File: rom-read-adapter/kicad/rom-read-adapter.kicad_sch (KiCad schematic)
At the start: 51 parts, among them J1 Host_Conn_02x25, J10 Conn_01x04_Pin, J2 ZIF-48, J3 Conn_01x24_Pin, J4 Conn_01x13_Pin, J5 Conn_01x05_Pin

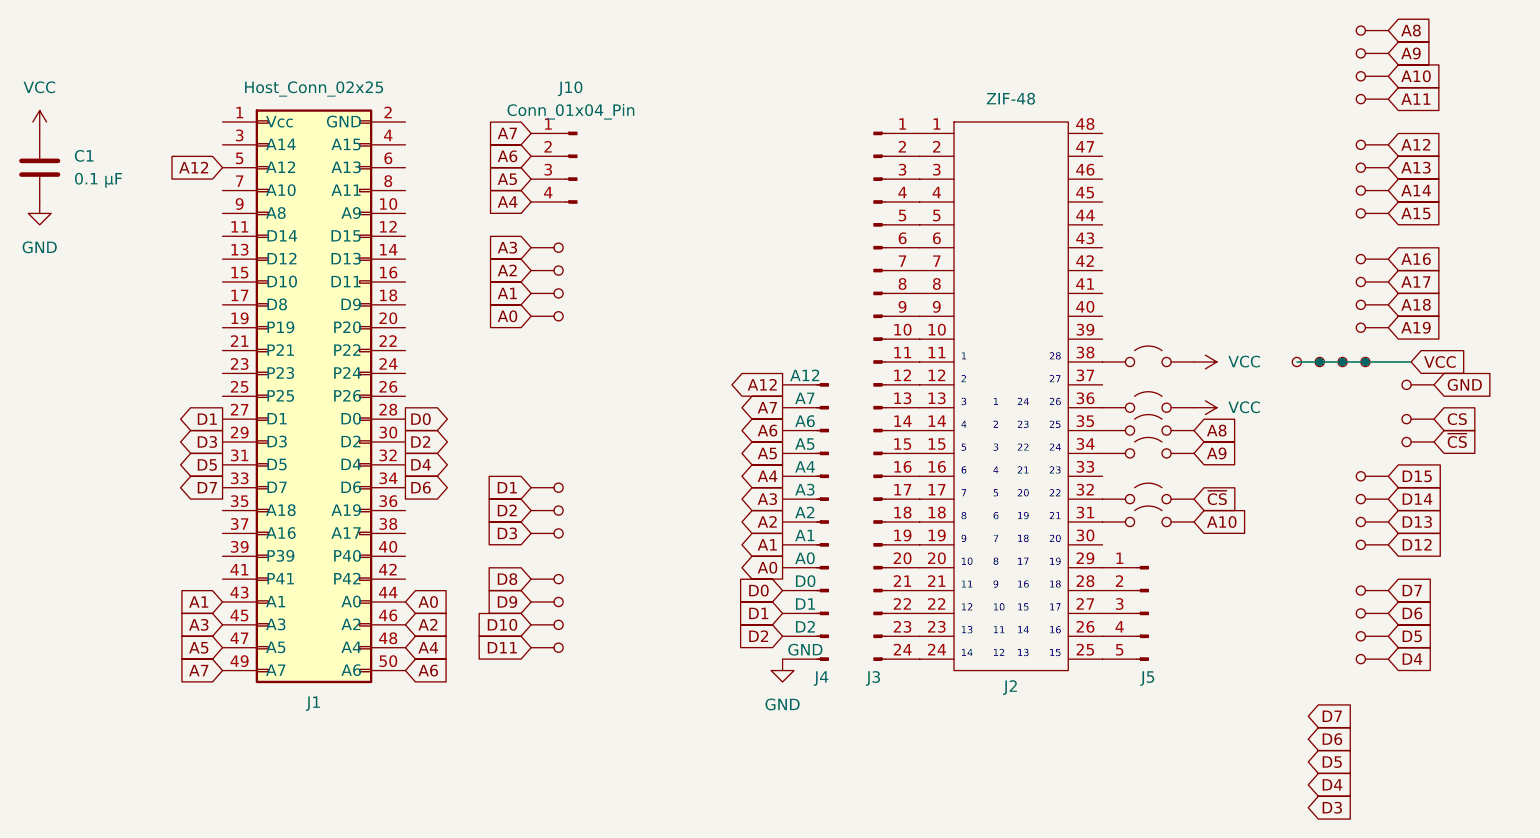
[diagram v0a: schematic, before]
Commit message: WIP rom-read-adapter sch: Added J6.
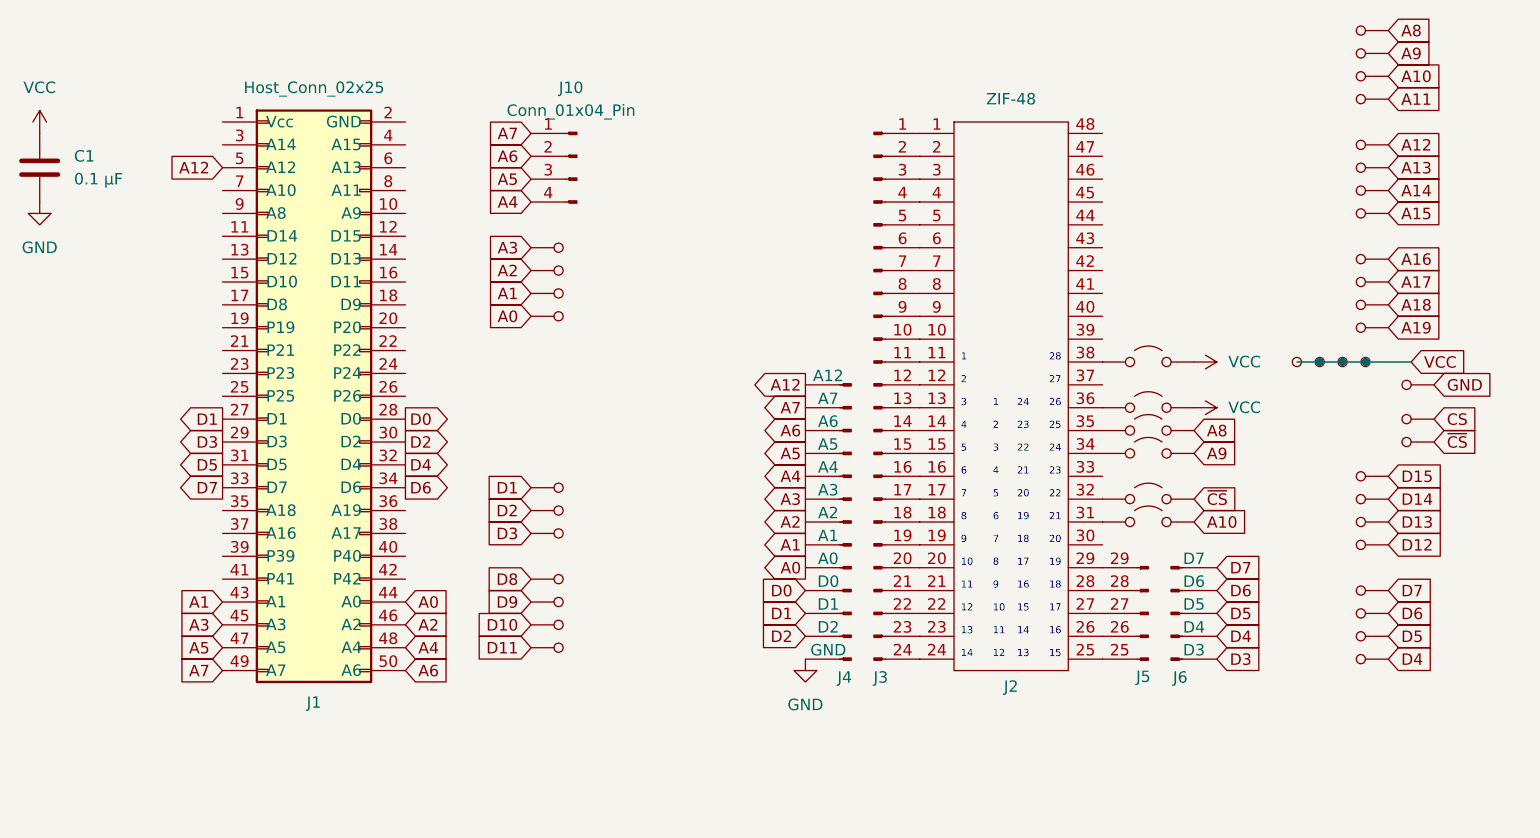
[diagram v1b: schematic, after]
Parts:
- added J6: Conn_01x05_Pin, symbol Connector:Conn_01x05_Pin
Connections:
- net D3: now also J6.1 (D3)
- net D4: now also J6.2 (D4)
- net D5: now also J6.3 (D5)
- net D6: now also J6.4 (D6)
- net D7: now also J6.5 (D7)
- net at J2., J2.28: now also J5.28 (Pin_4); no longer J5.2 (Pin_2)
- net at J2.25: now also J5.25 (Pin_1); no longer J5.5 (Pin_5)
- net at J2.26: now also J5.26 (Pin_2); no longer J5.4 (Pin_4)
- net at J2.27: now also J5.27 (Pin_3); no longer J5.3 (Pin_3)
- net at J2.29: now also J5.29 (Pin_5); no longer J5.1 (Pin_1)
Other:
- moved on the sheet: J4, J5
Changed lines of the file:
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@@
 	(global_label "A7"
 		(shape output)
-		(at 113.03 95.25 180)
+		(at 115.57 95.25 180)
 		(fields_autoplaced yes)
 		(effects
@@
 		)
 		(property "Intersheetrefs" "${INTERSHEET_REFS}"
-			(at 107.7467 95.25 0)
+			(at 110.2867 95.25 0)
 			(effects
 				(font
@@
 	(global_label "A2"
 		(shape output)
-		(at 113.03 107.95 180)
+		(at 115.57 107.95 180)
 		(fields_autoplaced yes)
 		(effects
@@
 		)
 		(property "Intersheetrefs" "${INTERSHEET_REFS}"
-			(at 107.7467 107.95 0)
+			(at 110.2867 107.95 0)
 			(effects
 				(font
@@
 	(global_label "D3"
 		(shape input)
-		(at 171.45 139.7 0)
+		(at 161.29 123.19 0)
 		(fields_autoplaced yes)
 		(effects
@@
 		)
 		(property "Intersheetrefs" "${INTERSHEET_REFS}"
-			(at 176.9147 139.7 0)
+			(at 166.7547 123.19 0)
 			(effects
 				(font
@@
 	(global_label "A12"
 		(shape output)
-		(at 113.03 92.71 180)
+		(at 115.57 92.71 180)
 		(fields_autoplaced yes)
 		(effects
@@
 		)
 		(property "Intersheetrefs" "${INTERSHEET_REFS}"
-			(at 106.5372 92.71 0)
+			(at 109.0772 92.71 0)
 			(effects
 				(font
@@
 	(global_label "D2"
 		(shape input)
-		(at 113.03 120.65 180)
+		(at 115.57 120.65 180)
 		(fields_autoplaced yes)
 		(effects
@@
 		)
 		(property "Intersheetrefs" "${INTERSHEET_REFS}"
-			(at 107.5653 120.65 0)
+			(at 110.1053 120.65 0)
 			(effects
 				(font
@@
 	(global_label "D1"
 		(shape input)
-		(at 113.03 118.11 180)
+		(at 115.57 118.11 180)
 		(fields_autoplaced yes)
 		(effects
@@
 		)
 		(property "Intersheetrefs" "${INTERSHEET_REFS}"
-			(at 107.5653 118.11 0)
+			(at 110.1053 118.11 0)
 			(effects
 				(font
@@
 	(global_label "A0"
 		(shape output)
-		(at 113.03 113.03 180)
+		(at 115.57 113.03 180)
 		(fields_autoplaced yes)
 		(effects
@@
 		)
 		(property "Intersheetrefs" "${INTERSHEET_REFS}"
-			(at 107.7467 113.03 0)
+			(at 110.2867 113.03 0)
 			(effects
 				(font
@@
 	(global_label "A5"
 		(shape output)
-		(at 113.03 100.33 180)
+		(at 115.57 100.33 180)
 		(fields_autoplaced yes)
 		(effects
@@
 		)
 		(property "Intersheetrefs" "${INTERSHEET_REFS}"
-			(at 107.7467 100.33 0)
+			(at 110.2867 100.33 0)
 			(effects
 				(font
@@
 	(global_label "D4"
 		(shape input)
-		(at 171.45 137.16 0)
+		(at 161.29 120.65 0)
 		(fields_autoplaced yes)
 		(effects
@@
 		)
 		(property "Intersheetrefs" "${INTERSHEET_REFS}"
-			(at 176.9147 137.16 0)
+			(at 166.7547 120.65 0)
 			(effects
 				(font
@@
 	(global_label "A1"
 		(shape output)
-		(at 113.03 110.49 180)
+		(at 115.57 110.49 180)
 		(fields_autoplaced yes)
 		(effects
@@
 		)
 		(property "Intersheetrefs" "${INTERSHEET_REFS}"
-			(at 107.7467 110.49 0)
+			(at 110.2867 110.49 0)
 			(effects
 				(font
@@
 	(global_label "A3"
 		(shape output)
-		(at 113.03 105.41 180)
+		(at 115.57 105.41 180)
 		(fields_autoplaced yes)
 		(effects
@@
 		)
 		(property "Intersheetrefs" "${INTERSHEET_REFS}"
-			(at 107.7467 105.41 0)
+			(at 110.2867 105.41 0)
 			(effects
 				(font
@@
 	(global_label "D5"
 		(shape input)
-		(at 171.45 134.62 0)
+		(at 161.29 118.11 0)
 		(fields_autoplaced yes)
 		(effects
@@
 		)
 		(property "Intersheetrefs" "${INTERSHEET_REFS}"
-			(at 176.9147 134.62 0)
+			(at 166.7547 118.11 0)
 			(effects
 				(font
@@
 	(global_label "A6"
 		(shape output)
-		(at 113.03 97.79 180)
+		(at 115.57 97.79 180)
 		(fields_autoplaced yes)
 		(effects
@@
 		)
 		(property "Intersheetrefs" "${INTERSHEET_REFS}"
-			(at 107.7467 97.79 0)
+			(at 110.2867 97.79 0)
 			(effects
 				(font
@@
 	(global_label "D6"
 		(shape input)
-		(at 171.45 132.08 0)
+		(at 161.29 115.57 0)
 		(fields_autoplaced yes)
 		(effects
@@
 		)
 		(property "Intersheetrefs" "${INTERSHEET_REFS}"
-			(at 176.9147 132.08 0)
+			(at 166.7547 115.57 0)
 			(effects
 				(font
@@
 	(global_label "D7"
 		(shape input)
-		(at 171.45 129.54 0)
+		(at 161.29 113.03 0)
 		(fields_autoplaced yes)
 		(effects
@@
 		)
 		(property "Intersheetrefs" "${INTERSHEET_REFS}"
-			(at 176.9147 129.54 0)
+			(at 166.7547 113.03 0)
 			(effects
 				(font
@@
 	(global_label "A4"
 		(shape output)
-		(at 113.03 102.87 180)
+		(at 115.57 102.87 180)
 		(fields_autoplaced yes)
 		(effects
@@
 		)
 		(property "Intersheetrefs" "${INTERSHEET_REFS}"
-			(at 107.7467 102.87 0)
+			(at 110.2867 102.87 0)
 			(effects
 				(font
@@
 	(global_label "D0"
 		(shape input)
-		(at 113.03 115.57 180)
+		(at 115.57 115.57 180)
 		(fields_autoplaced yes)
 		(effects
@@
 		)
 		(property "Intersheetrefs" "${INTERSHEET_REFS}"
-			(at 107.5653 115.57 0)
+			(at 110.1053 115.57 0)
 			(effects
 				(font
@@
 	(symbol
 		(lib_id "power:GND")
-		(at 113.03 123.19 0)
+		(at 115.57 123.19 0)
 		(unit 1)
 		(exclude_from_sim no)
@@
 		(fields_autoplaced yes)
 		(property "Reference" "#PWR03"
-			(at 113.03 129.54 0)
+			(at 115.57 129.54 0)
 			(effects
 				(font
@@
 		)
 		(property "Value" "GND"
-			(at 113.03 128.27 0)
+			(at 115.57 128.27 0)
 			(effects
 				(font
@@
 		)
 		(property "Footprint" ""
-			(at 113.03 123.19 0)
+			(at 115.57 123.19 0)
 			(effects
 				(font
@@
 		)
 		(property "Datasheet" ""
-			(at 113.03 123.19 0)
+			(at 115.57 123.19 0)
 			(effects
 				(font
@@
 		)
 		(property "Description" "Power symbol creates a global label with name \"GND\" , ground"
-			(at 113.03 123.19 0)
+			(at 115.57 123.19 0)
 			(effects
 				(font
@@
 	)
 	(symbol
+		(lib_name "Conn_01x05_Pin_1")
 		(lib_id "Connector:Conn_01x05_Pin")
-		(at 153.67 118.11 0)
-		(mirror y)
+		(at 153.67 118.11 180)
 		(unit 1)
 		(exclude_from_sim no)
@@
 		(dnp no)
 		(property "Reference" "J5"
-			(at 153.67 125.222 0)
+			(at 153.1231 125.1429 0)
 			(effects
 				(font
@@
 		)
 		(property "Value" "Conn_01x05_Pin"
-			(at 153.035 110.49 0)
+			(at 153.035 125.73 0)
 			(effects
 				(font
@@
 			)
 		)
-		(pin "5"
+		(pin "27"
 		)
-		(pin "2"
+		(pin "29"
 		)
-		(pin "1"
+		(pin "25"
 		)
-		(pin "3"
+		(pin "26"
 		)
-		(pin "4"
+		(pin "28"
 		)
 		(instances
@@
 	(symbol
 		(lib_id "Connector:Conn_01x13_Pin")
-		(at 118.11 107.95 0)
+		(at 120.65 107.95 0)
 		(mirror y)
 		(unit 1)
@@
 		(dnp no)
 		(property "Reference" "J4"
-			(at 116.586 125.222 0)
+			(at 119.126 125.222 0)
 			(effects
 				(font
@@
 		)
 		(property "Value" "Conn_01x13_Pin"
-			(at 119.38 109.2199 0)
+			(at 121.92 109.2199 0)
 			(effects
 				(font
@@
 		)
 		(property "Footprint" ""
-			(at 118.11 107.95 0)
+			(at 120.65 107.95 0)
 			(effects
 				(font
@@
 		)
 		(property "Datasheet" "~"
-			(at 118.11 107.95 0)
+			(at 120.65 107.95 0)
 			(effects
 				(font
@@
 		)
 		(property "Description" "Generic connector, single row, 01x13, script generated"
-			(at 122.174 88.138 0)
+			(at 124.714 88.138 0)
 			(effects
 				(font
@@
 		(dnp no)
 		(property "Reference" "J3"
-			(at 123.19 125.222 0)
+			(at 123.952 125.222 0)
 			(effects
 				(font
@@
 					(unit 1)
 				)
+			)
+		)
+	)
+	(symbol
+		(lib_id "Connector:Conn_01x05_Pin")
+		(at 156.21 118.11 0)
+		(mirror x)
+		(unit 1)
+		(exclude_from_sim no)
+		(in_bom yes)
+		(on_board yes)
+		(dnp no)
+		(property "Reference" "J6"
+			(at 157.226 125.222 0)
+			(effects
+				(font
+					(size 1.27 1.27)
+				)
+			)
+		)
+		(property "Value" "Conn_01x05_Pin"
+			(at 156.845 125.73 0)
+			(effects
+				(font
+					(size 1.27 1.27)
+				)
+				(hide yes)
+			)
+		)
+		(property "Footprint" ""
+			(at 156.21 118.11 0)
+			(effects
+				(font
+					(size 1.27 1.27)
+				)
+				(hide yes)
+			)
+		)
+		(property "Datasheet" "~"
+			(at 156.21 118.11 0)
+			(effects
+				(font
+					(size 1.27 1.27)
+				)
+				(hide yes)
+			)
+		)
+		(property "Description" "Generic connector, single row, 01x05, script generated"
+			(at 157.988 106.68 0)
+			(effects
+				(font
+					(size 1.27 1.27)
+				)
+				(hide yes)
+			)
+		)
+		(pin "3"
+		)
+		(pin "5"
+		)
+		(pin "2"
+		)
+		(pin "4"
+		)
+		(pin "1"
+		)
+		(instances
+			(project ""
+				(path "/65bf6d13-0c24-4e8f-8a57-e3ae2776eac6"
+					(reference "J6")
+					(unit 1)
+				)
